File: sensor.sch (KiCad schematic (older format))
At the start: 82 parts, among them CON1 Micro USB, CON2 PROG, CON3 Jack-DC, Q1 BSS214N, Q2 BSS214N, Q3 BSS214N, Q4 BSS214N, Q5 BSS214N, Q6 BSS214N, SW1 RESET, SW2 CFG, U1 LM7805, U2 TLV1117LV33DCY, U3 ESP-12F, U4 HTU21D, U5 PMS7003

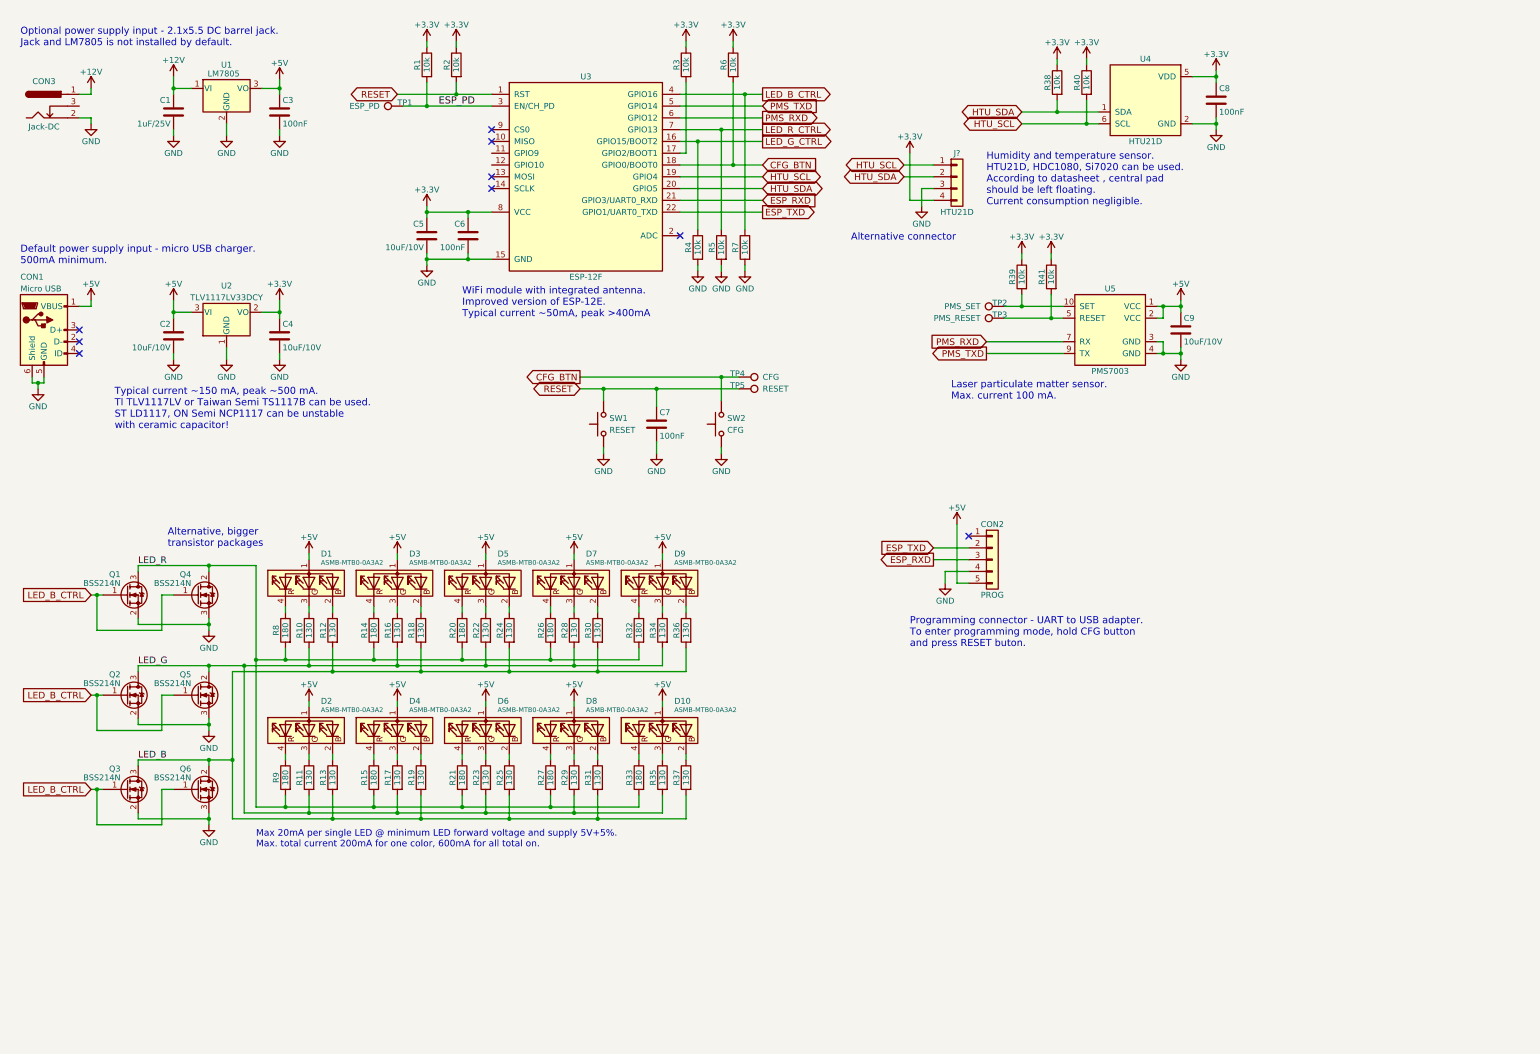
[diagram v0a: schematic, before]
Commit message: Schematic finishing and cleanup.
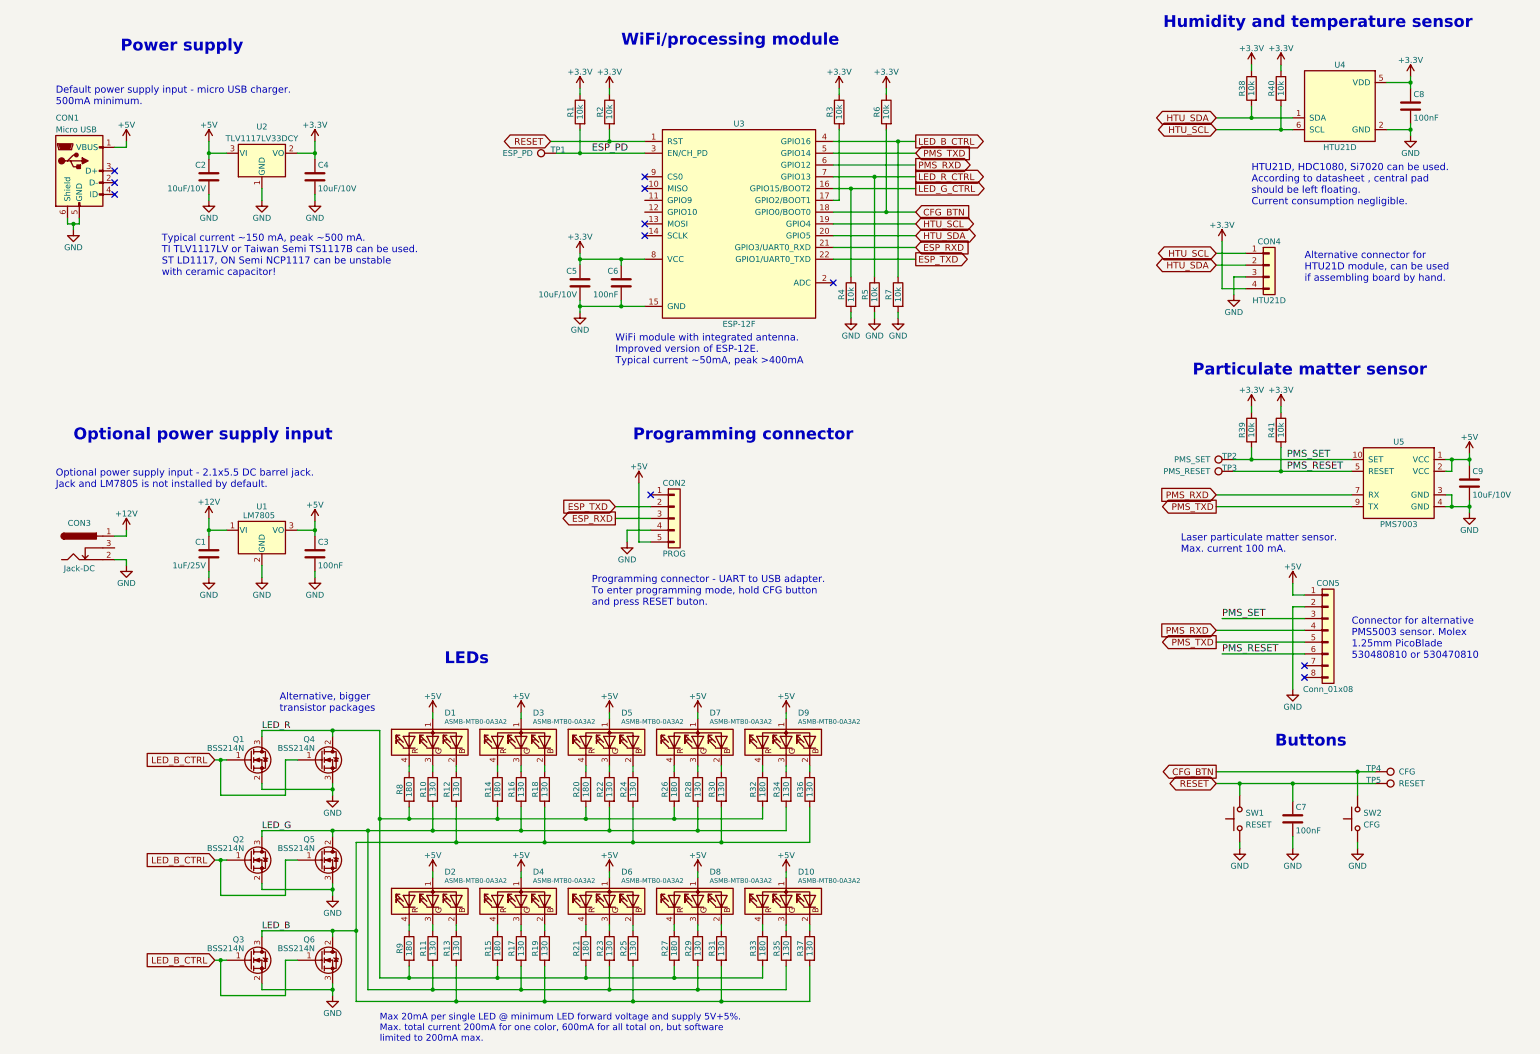
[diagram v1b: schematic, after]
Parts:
- added CON5: Conn_01x08, Connectors_Molex:Molex_PicoBlade_53048-0810_08x1.25mm_Angled, symbol Conn_01x08
- CON2: footprint Pin_Headers:Pin_Header_Angled_1x05_Pitch2.54mm -> Pin_Headers:Pin_Header_Straight_1x05_Pitch2.54mm
- CON3: footprint (none) -> Connectors:BARREL_JACK
- CON4: renamed from J?; footprint (none) -> Pin_Headers:Pin_Header_Straight_1x04_Pitch2.54mm
- SW1, SW2: footprint (none) -> Buttons_Switches_SMD:SW_SPST_EVQQ2
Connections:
- net +5V: now also CON5.1 (Pin_1)
- net GND: now also CON5.2 (Pin_2)
- net PMS_RXD: now also CON5.4 (Pin_4)
- net PMS_TXD: now also CON5.5 (Pin_5)
- net PMS_SET: now reaches R39.2, TP2.1, U5.10 (SET)
- net PMS_SET: now also CON5.3 (Pin_3)
- net PMS_RESET: now reaches R41.2, TP3.1, U5.5 (RESET)
- net PMS_RESET: now also CON5.6 (Pin_6)
- no-connect marks 9 -> 11
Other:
- note added: "Alternative connector for \nHTU21D module, can be used\nif assembling board by hand."
- note added: "Buttons"
- note added: "Connector for alternative\nPMS5003 sensor. Molex\n1.25mm PicoBlade\n530480810 or 530470810"
- note added: "HTU21D, HDC1080, Si7020 can be used.\nAccording to datasheet , central pad \nshould be left floating.\nCurrent consumption negligible."
- note added: "Humidity and temperature sensor"
- note added: "LEDs"
- note added: "Max 20mA per single LED @ minimum LED forward voltage and supply 5V+5%.\nMax. total current 200mA for one color, 600mA for all total on, but software\nlimited to 200mA max."
- note added: "Optional power supply input"
- note added: "Particulate matter sensor"
- note added: "Power supply"
- note added: "Programming connector"
- note added: "WiFi/processing module"
- note removed: "Alternative connector"
- note removed: "Humidity and temperature sensor.\nHTU21D, HDC1080, Si7020 can be used.\nAccording to datasheet , central pad \nshould be left floating.\nCurrent consumption negligible."
- note removed: "Max 20mA per single LED @ minimum LED forward voltage and supply 5V+5%.\nMax. total current 200mA for one color, 600mA for all total on."
- moved on the sheet: C1, C2, C3, C4, C5, C6, C7, C8, C9, CON1, CON2, CON3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
